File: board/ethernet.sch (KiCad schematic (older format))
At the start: 1 part

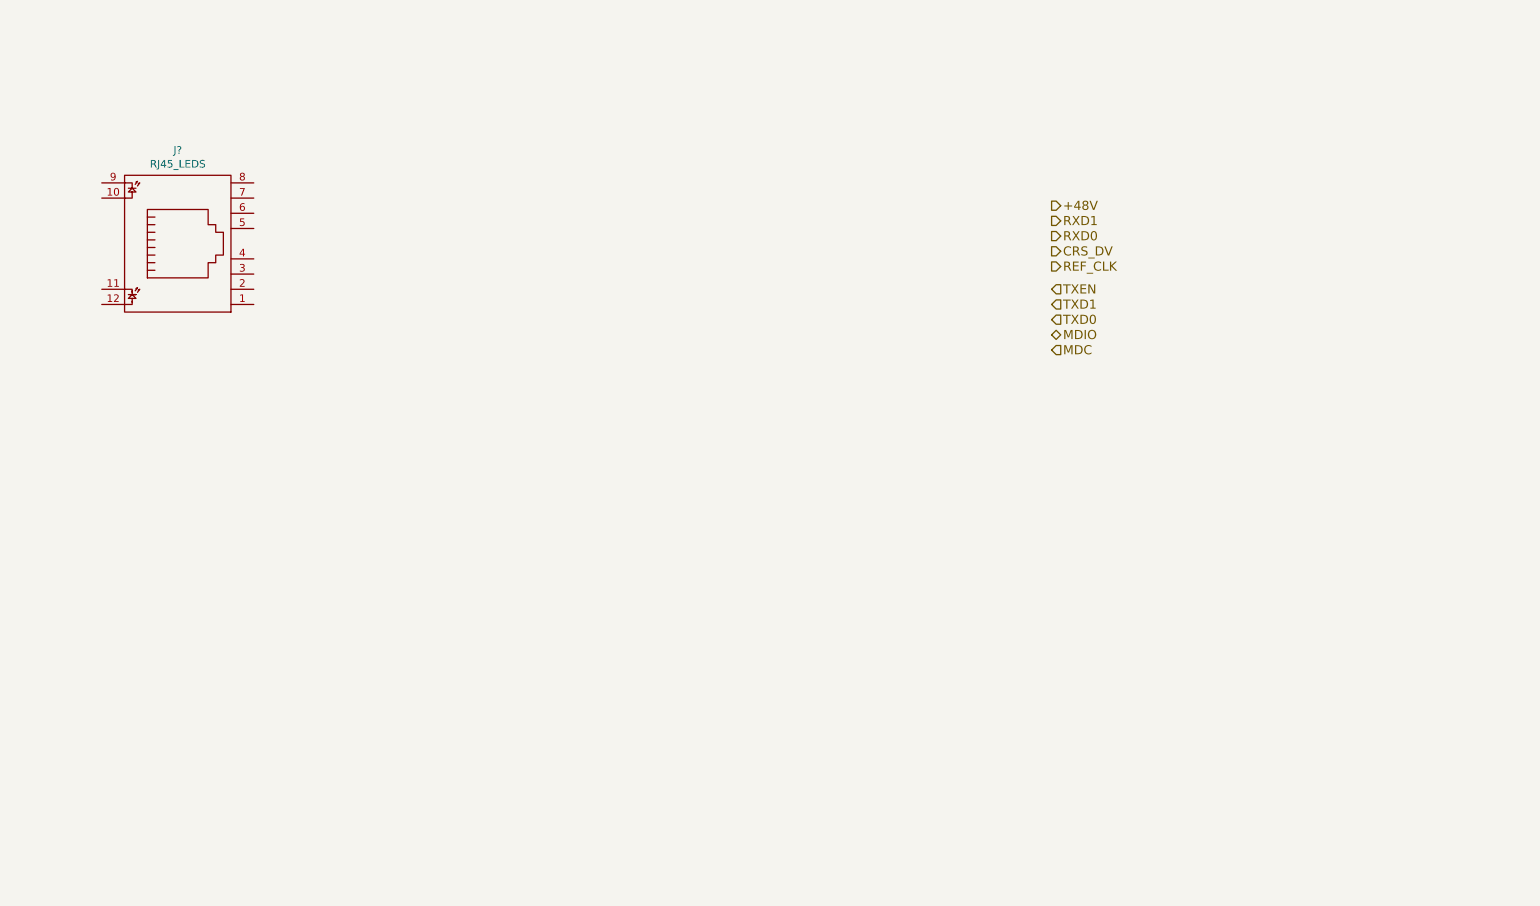
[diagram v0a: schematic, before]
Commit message: Roughed out ethernet sheet
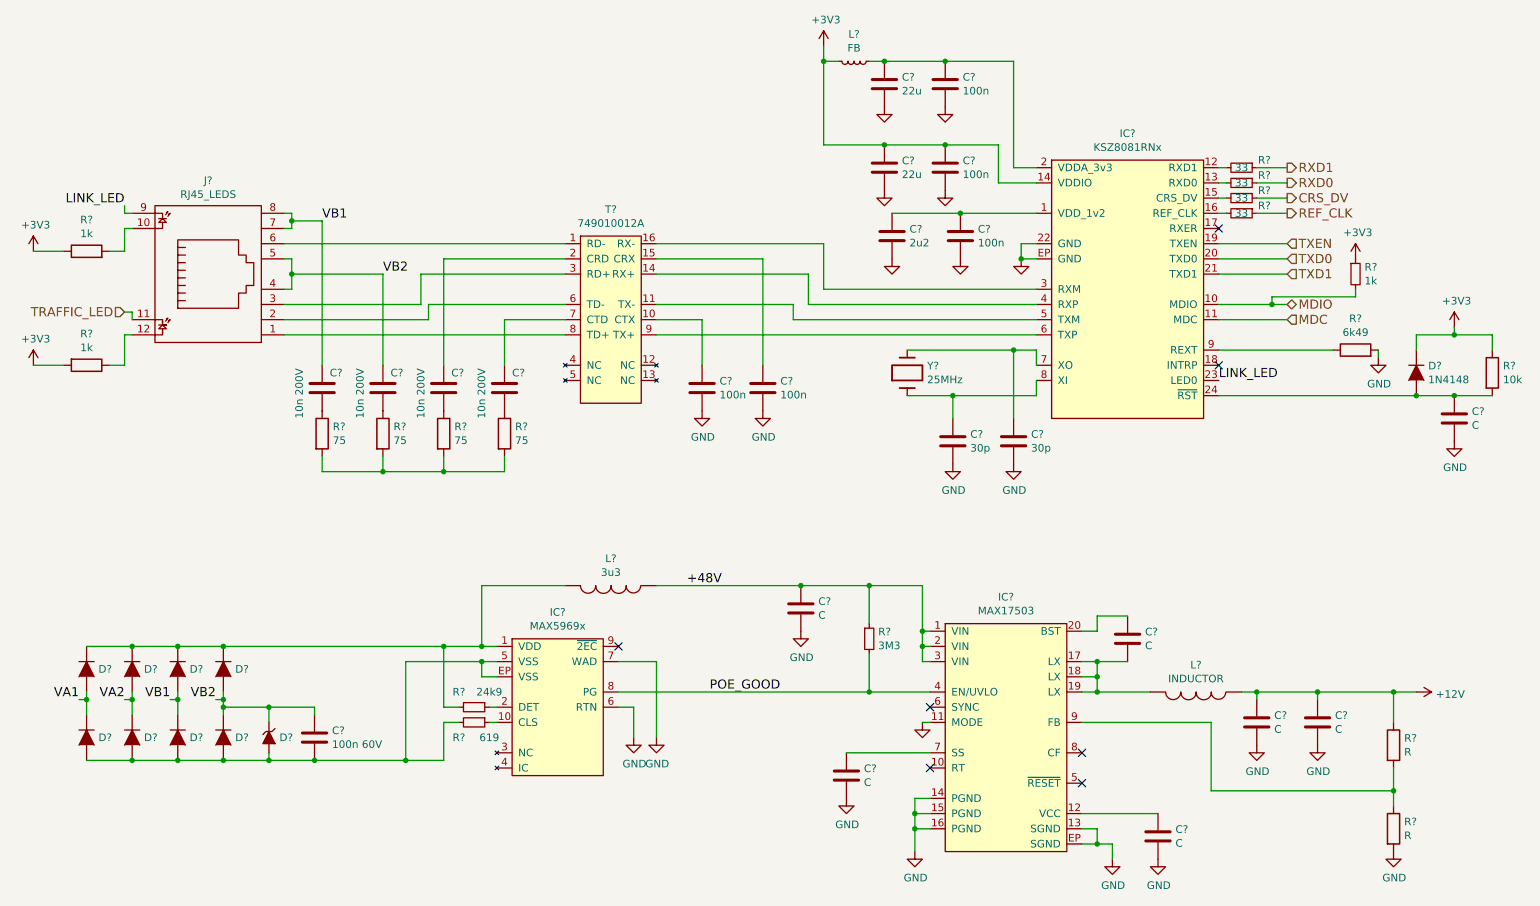
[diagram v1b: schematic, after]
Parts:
- added C? (x4): 10n 200V, agg:0805, symbol C
- added C? (x5): 100n, agg:0603, symbol C
- added C? (x2): 30p, agg:0603, symbol C
- added C?: 2u2, agg:0603, symbol C
- added C? (x2): 22u, agg:1206, symbol C
- added C?: C, agg:0603, symbol C
- added C?: 100n 60V, agg:0805, symbol C
- added C? (x6): C, symbol C
- added D?: 1N4148, agg:SOD-323, symbol D
- added D? (x8): SS110B, agg:DO-214AA-SMB, symbol D
- added D?: SMAJ58A, agg:DO-214AC-SMA, symbol ZENERsmall
- added IC?: KSZ8081RNx, agg:QFN-24-EP-MICREL, symbol KSZ8081RNx
- added IC?: MAX5969x, agg:DFN-10-EP-MAX, symbol MAX5969x
- added IC?: MAX17503, agg:QFN-20-EP-MAX, symbol MAX17503
- added L?: FB, agg:0603, symbol L_Small
- added L?: 3u3, symbol INDUCTOR
- added L?: INDUCTOR, symbol INDUCTOR
- added R? (x4): 75, agg:0603, symbol R
- added R? (x4): 33, agg:0603, symbol R_Small
- added R?: 1k, agg:0603, symbol R_Small
- added R?: 6k49, agg:0603, symbol R
- added R?: 10k, agg:0603, symbol R
- added R? (x2): 1k, agg:0603, symbol R
- added R?: 24k9, agg:0603, symbol R_Small
- added R?: 619, agg:0603, symbol R_Small
- added R?: 3M3, symbol R_Small
- added R? (x2): R, symbol R
- added T?: 749010012A, agg:749010012A, symbol 749010012A
- added Y?: 25MHz, agg:XTAL-50x32, symbol Crystal
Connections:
- net +48V: now also C?.1, IC?.1 (VIN), IC?.2 (VIN), IC?.3 (VIN), L?.1, R?.1
- net CRS_DV: now also R?.1
- net MDC: now also IC?.11 (MDC)
- net MDIO: now also IC?.10 (MDIO), R?.2
- net REF_CLK: now also R?.1
- net RXD0: now also R?.1
- net RXD1: now also R?.1
- net TXD0: now also IC?.20 (TXD0)
- net TXD1: now also IC?.21 (TXD1)
- net TXEN: now also IC?.19 (TXEN)
- net at J?.1: now also T?.8 (TD+)
- net at J?.10: now also R?.2
- net TRAFFIC_LED: now reaches J?.11
- net at J?.12: now also R?.1
- net at J?.2: now also T?.6 (TD-)
- net at J?.3: now also T?.3 (RD+)
- net VB2: now reaches J?.4
- net VB2: now also J?.5, C?.1, C?.1, D?.1 (K), D?.1 (K), D?.2 (A)
- net at J?.6: now also T?.1 (RD-)
- net VB1: now reaches J?.7
- net VB1: now also J?.8, C?.1, D?.1 (K), D?.2 (A)
- net LINK_LED: now reaches J?.9
- net LINK_LED: now also IC?.23 (LED0)
- new net: C?.1, T?.10 (CTX)
- new net: IC?.5 (TXM), T?.11 (TX-)
- new net: IC?.4 (RXP), T?.14 (RX+)
- new net: C?.1, T?.15 (CRX)
- new net: IC?.3 (RXM), T?.16 (RX-)
- new net: C?.1, T?.2 (CRD)
- new net: C?.1, T?.7 (CTD)
- new net: IC?.6 (TXP), T?.9 (TX+)
- new net: C?.1, C?.1, IC?.1 (VDD_1v2)
- new net: IC?.12 (RXD1), R?.2
- new net: IC?.13 (RXD0), R?.2
- new net: IC?.15 (CRS_DV), R?.2
- new net: IC?.16 (REF_CLK), R?.2
- new net: C?.1, C?.1, IC?.2 (VDDA_3v3), L?.1
- new net: C?.1, D?.2 (A), IC?.24 (~RST), R?.2
- new net: C?.1, IC?.7 (XO), Y?.2
- new net: C?.1, IC?.8 (XI), Y?.1
- new net: IC?.9 (REXT), R?.1
- new net: D?.1 (K), D?.1 (K), D?.1 (K), D?.1 (K), IC?.1 (VDD), L?.2, R?.2
- new net: IC?.10 (CLS), R?.1
- new net: IC?.2 (DET), R?.1
- new net: C?.2, D?.2 (A), D?.2 (A), D?.2 (A), D?.2 (A), D?.2 (A), IC?.5 (VSS), IC?.EP (VSS), R?.2
- new net: C?.1, IC?.12 (VCC)
- new net: C?.2, IC?.17 (LX), IC?.18 (LX), IC?.19 (LX), L?.2
- new net: C?.1, IC?.20 (BST)
- new net: C?.1, IC?.7 (SS)
- new net: IC?.9 (FB), R?.1, R?.2
- new net: C?.2, R?.1 (x4)
- new net: R?.2, R?.2, R?.2, R?.2
- new net +12V: C?.1, C?.1, L?.1, R?.1
- new net +3V3: C?.1, C?.1, D?.1 (K), IC?.14 (VDDIO), L?.2, R?.1, R?.1, R?.1, R?.2
- new net GND: C?.2, C?.2, C?.2, C?.2, C?.2, C?.2, C?.2, C?.2, C?.2, C?.2, C?.2, C?.2, C?.2, C?.2, C?.2, C?.2, IC?.11 (MODE), IC?.13 (SGND), IC?.14 (PGND), IC?.15 (PGND), IC?.16 (PGND), IC?.22 (GND), IC?.6 (RTN), IC?.7 (WAD), IC?.EP (GND), IC?.EP (SGND), R?.2, R?.2
- new net POE_GOOD: IC?.4 (EN/UVLO), IC?.8 (PG), R?.2
- new net VA1: D?.1 (K), D?.2 (A)
- new net VA2: D?.1 (K), D?.2 (A)
- no-connect marks 0 -> 7
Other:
- moved on the sheet: J?
